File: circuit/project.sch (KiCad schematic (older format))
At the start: 0 parts

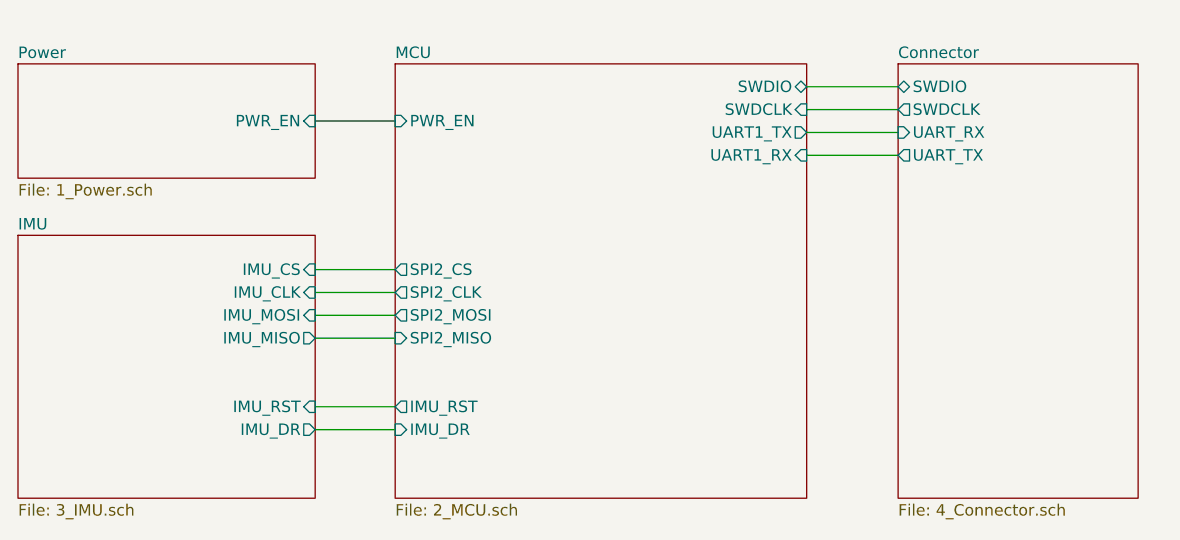
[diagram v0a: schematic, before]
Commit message: Added brushless motor communication interface and LCD control interface.
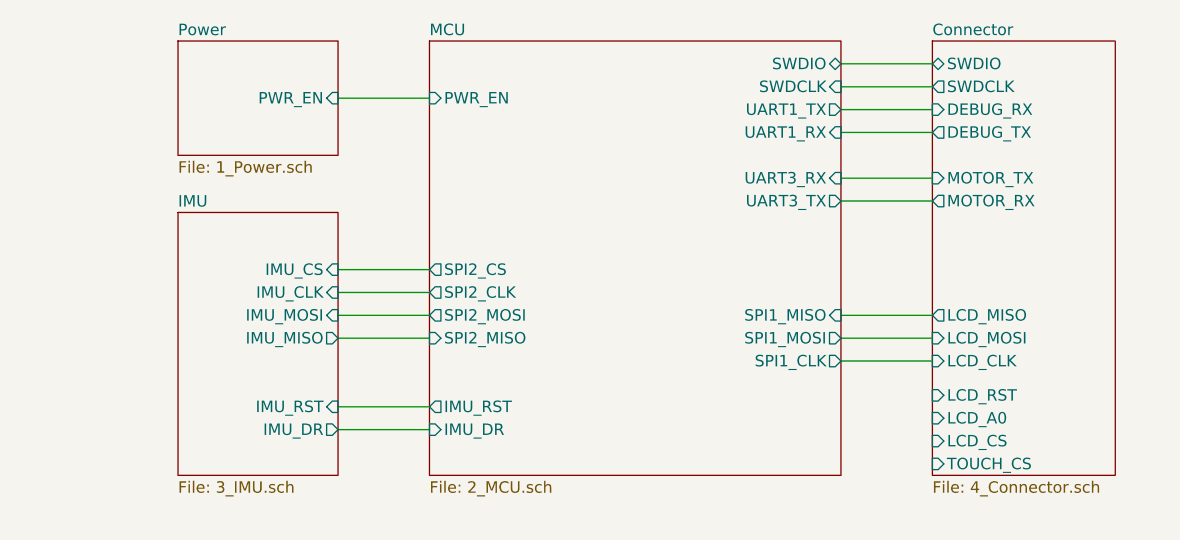
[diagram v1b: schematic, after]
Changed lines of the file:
@@
 $EndDescr
 $Sheet
-S 3150 3300 1300 500
+S 3850 3200 700  500
 U 6191448D
 F0 "Power" 50
 F1 "1_Power.sch" 50
-F2 "PWR_EN" I R 4450 3550 50
+F2 "PWR_EN" I R 4550 3450 50
 $EndSheet
 $Sheet
-S 4800 3300 1800 1900
+S 4950 3200 1800 1900
 U 6194FB75
 F0 "MCU" 50
 F1 "2_MCU.sch" 50
-F2 "PWR_EN" I L 4800 3550 50
-F3 "SPI2_CLK" O L 4800 4300 50
-F4 "SPI2_CS" O L 4800 4200 50
-F5 "SPI2_MISO" I L 4800 4500 50
-F6 "SPI2_MOSI" O L 4800 4400 50
-F7 "IMU_DR" I L 4800 4900 50
-F8 "IMU_RST" O L 4800 4800 50
-F9 "SWDIO" B R 6600 3400 50
-F10 "SWDCLK" I R 6600 3500 50
-F11 "UART1_TX" O R 6600 3600 50
-F12 "UART1_RX" I R 6600 3700 50
+F2 "PWR_EN" I L 4950 3450 50
+F3 "SPI2_CLK" O L 4950 4300 50
+F4 "SPI2_CS" O L 4950 4200 50
+F5 "SPI2_MISO" I L 4950 4500 50
+F6 "SPI2_MOSI" O L 4950 4400 50
+F7 "IMU_DR" I L 4950 4900 50
+F8 "IMU_RST" O L 4950 4800 50
+F9 "SWDIO" B R 6750 3300 50
+F10 "SWDCLK" I R 6750 3400 50
+F11 "UART1_TX" O R 6750 3500 50
+F12 "UART1_RX" I R 6750 3600 50
+F13 "UART3_TX" O R 6750 3900 50
+F14 "UART3_RX" I R 6750 3800 50
+F15 "SPI1_CLK" O R 6750 4600 50
+F16 "SPI1_MISO" I R 6750 4400 50
+F17 "SPI1_MOSI" O R 6750 4500 50
 $EndSheet
 $Sheet
-S 3150 4050 1300 1150
+S 3850 3950 700  1150
 U 61A493C9
 F0 "IMU" 50
 F1 "3_IMU.sch" 50
-F2 "IMU_CS" I R 4450 4200 50
-F3 "IMU_RST" I R 4450 4800 50
-F4 "IMU_DR" O R 4450 4900 50
-F5 "IMU_CLK" I R 4450 4300 50
-F6 "IMU_MOSI" I R 4450 4400 50
-F7 "IMU_MISO" O R 4450 4500 50
+F2 "IMU_CS" I R 4550 4200 50
+F3 "IMU_RST" I R 4550 4800 50
+F4 "IMU_DR" O R 4550 4900 50
+F5 "IMU_CLK" I R 4550 4300 50
+F6 "IMU_MOSI" I R 4550 4400 50
+F7 "IMU_MISO" O R 4550 4500 50
 $EndSheet
 Wire Wire Line
-	4450 3550 4800 3550
+	4550 3450 4950 3450
 $Sheet
-S 7000 3300 1050 1900
+S 7150 3200 800  1900
 U 61E2DD2B
 F0 "Connector" 50
 F1 "4_Connector.sch" 50
-F2 "SWDIO" B L 7000 3400 50
-F3 "SWDCLK" O L 7000 3500 50
-F4 "UART_TX" O L 7000 3700 50
-F5 "UART_RX" I L 7000 3600 50
+F2 "SWDIO" B L 7150 3300 50
+F3 "SWDCLK" O L 7150 3400 50
+F4 "LCD_CS" I L 7150 4950 50
+F5 "LCD_CLK" I L 7150 4600 50
+F6 "LCD_MOSI" I L 7150 4500 50
+F7 "LCD_A0" I L 7150 4850 50
+F8 "LCD_RST" I L 7150 4750 50
+F9 "LCD_MISO" O L 7150 4400 50
+F10 "TOUCH_CS" I L 7150 5050 50
+F11 "DEBUG_TX" O L 7150 3600 50
+F12 "DEBUG_RX" I L 7150 3500 50
+F13 "MOTOR_TX" I L 7150 3800 50
+F14 "MOTOR_RX" O L 7150 3900 50
 $EndSheet
 Wire Wire Line
-	4450 4200 4800 4200
+	4550 4200 4950 4200
 Wire Wire Line
-	4450 4300 4800 4300
+	4550 4300 4950 4300
 Wire Wire Line
-	4450 4400 4800 4400
+	4550 4400 4950 4400
 Wire Wire Line
-	4450 4500 4800 4500
+	4550 4500 4950 4500
 Wire Wire Line
-	4800 4800 4450 4800
+	4950 4800 4550 4800
 Wire Wire Line
-	4450 4900 4800 4900
+	4550 4900 4950 4900
 Wire Wire Line
-	6600 3400 7000 3400
+	6750 3300 7150 3300
 Wire Wire Line
-	7000 3500 6600 3500
+	7150 3400 6750 3400
 Wire Wire Line
-	6600 3600 7000 3600
+	6750 3500 7150 3500
 Wire Wire Line
-	7000 3700 6600 3700
+	7150 3600 6750 3600
+Wire Wire Line
+	6750 3800 7150 3800
+Wire Wire Line
+	6750 3900 7150 3900
+Wire Wire Line
+	6750 4400 7150 4400
+Wire Wire Line
+	6750 4500 7150 4500
+Wire Wire Line
+	6750 4600 7150 4600
 $EndSCHEMATC
